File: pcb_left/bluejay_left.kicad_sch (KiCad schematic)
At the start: 81 parts, among them J1 SJ-43514, U1 ATmega328P-PU, Y1 16MHz

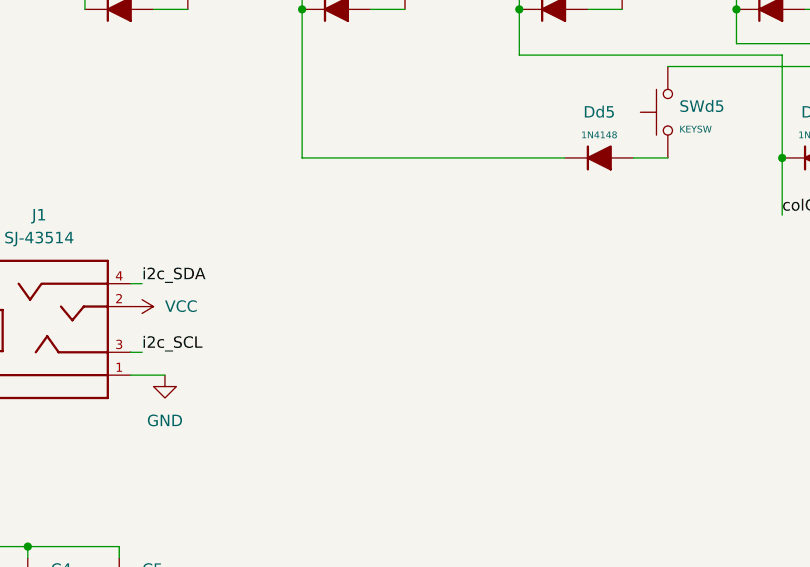
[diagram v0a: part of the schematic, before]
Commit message: Fine tune pcbs
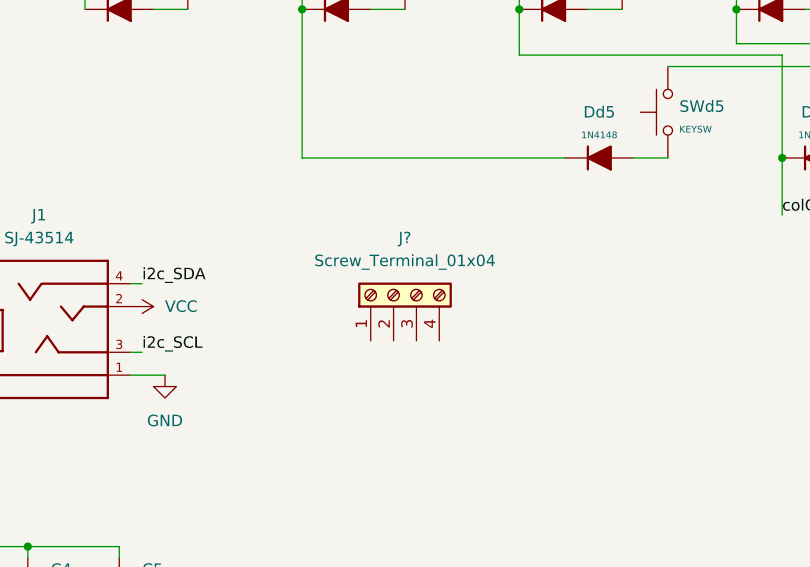
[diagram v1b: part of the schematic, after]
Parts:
- added J?: Screw_Terminal_01x04, symbol Connector:Screw_Terminal_01x04
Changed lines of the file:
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@@
     (pin "2")
+  )
+  (symbol (lib_id "Connector:Screw_Terminal_01x04") (at 144.78 156.21 90) (unit 1)
+    (in_bom yes) (on_board yes) (fields_autoplaced)
+    (property "Reference" "J?" (id 0) (at 146.05 149.86 90))
+    (property "Value" "Screw_Terminal_01x04" (id 1) (at 146.05 152.4 90))
+    (property "Footprint" "" (id 2) (at 144.78 156.21 0)
+      (effects (font (size 1.27 1.27)) hide)
+    )
+    (property "Datasheet" "~" (id 3) (at 144.78 156.21 0)
+      (effects (font (size 1.27 1.27)) hide)
+    )
+    (pin "1")
+    (pin "2")
+    (pin "3")
+    (pin "4")
   )
   (symbol (lib_id "Diode_AKL:1N4148") (at 138.43 86.36 180) (unit 1)
@@
       (reference "J1") (unit 1) (value "SJ-43514") (footprint "BlueJay footprints:CUI_SJ-43514")
     )
+    (path "/1447b0b5-ab38-407e-b41f-aa727794d4da"
+      (reference "J?") (unit 1) (value "Screw_Terminal_01x04") (footprint "")
+    )
     (path "/31642483-9c10-4ba0-a4b2-91eb418caf17"

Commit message: Produce test gerber files
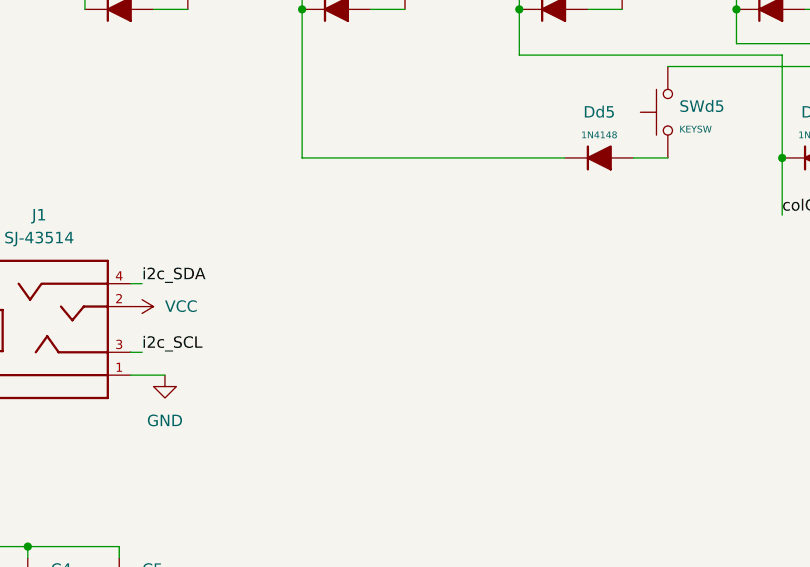
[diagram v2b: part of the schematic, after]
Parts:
- removed J?: Screw_Terminal_01x04, symbol Connector:Screw_Terminal_01x04
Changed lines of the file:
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@@
     (pin "2")
-  )
-  (symbol (lib_id "Connector:Screw_Terminal_01x04") (at 144.78 156.21 90) (unit 1)
-    (in_bom yes) (on_board yes) (fields_autoplaced)
-    (property "Reference" "J?" (id 0) (at 146.05 149.86 90))
-    (property "Value" "Screw_Terminal_01x04" (id 1) (at 146.05 152.4 90))
-    (property "Footprint" "" (id 2) (at 144.78 156.21 0)
-      (effects (font (size 1.27 1.27)) hide)
-    )
-    (property "Datasheet" "~" (id 3) (at 144.78 156.21 0)
-      (effects (font (size 1.27 1.27)) hide)
-    )
-    (pin "1")
-    (pin "2")
-    (pin "3")
-    (pin "4")
   )
   (symbol (lib_id "Diode_AKL:1N4148") (at 138.43 86.36 180) (unit 1)
@@
       (reference "J1") (unit 1) (value "SJ-43514") (footprint "BlueJay footprints:CUI_SJ-43514")
     )
-    (path "/1447b0b5-ab38-407e-b41f-aa727794d4da"
-      (reference "J?") (unit 1) (value "Screw_Terminal_01x04") (footprint "")
-    )
     (path "/31642483-9c10-4ba0-a4b2-91eb418caf17"
